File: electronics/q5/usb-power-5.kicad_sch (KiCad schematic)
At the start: 4 parts, among them U2 Li-ion charger, U3 3.20481V adjustable LDO, U7 System soft-power latch switch

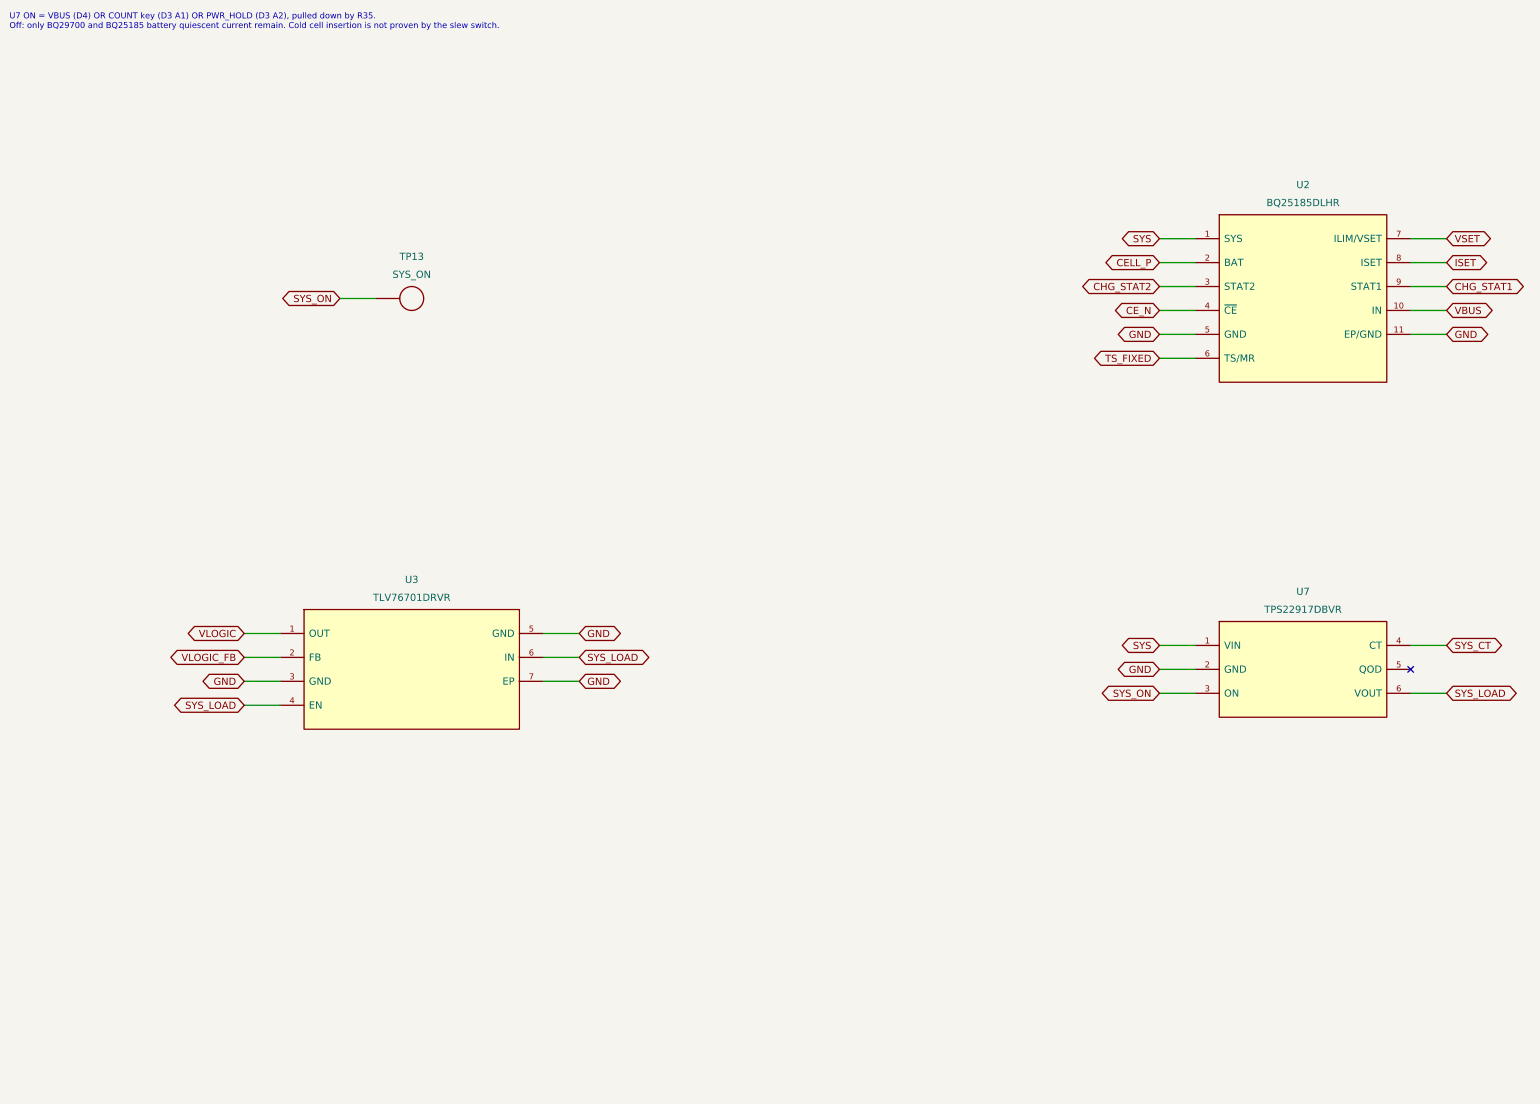
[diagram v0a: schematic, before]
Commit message: WIP: Q5 design-lock routing iteration snapshot (not verified)
Co-Authored-By: Claude Opus 5.5 <noreply@anthropic.com>
Claude-Session: https://claude.ai/code/session_01UrkzLMrBi6iLPSL5SbMCA7
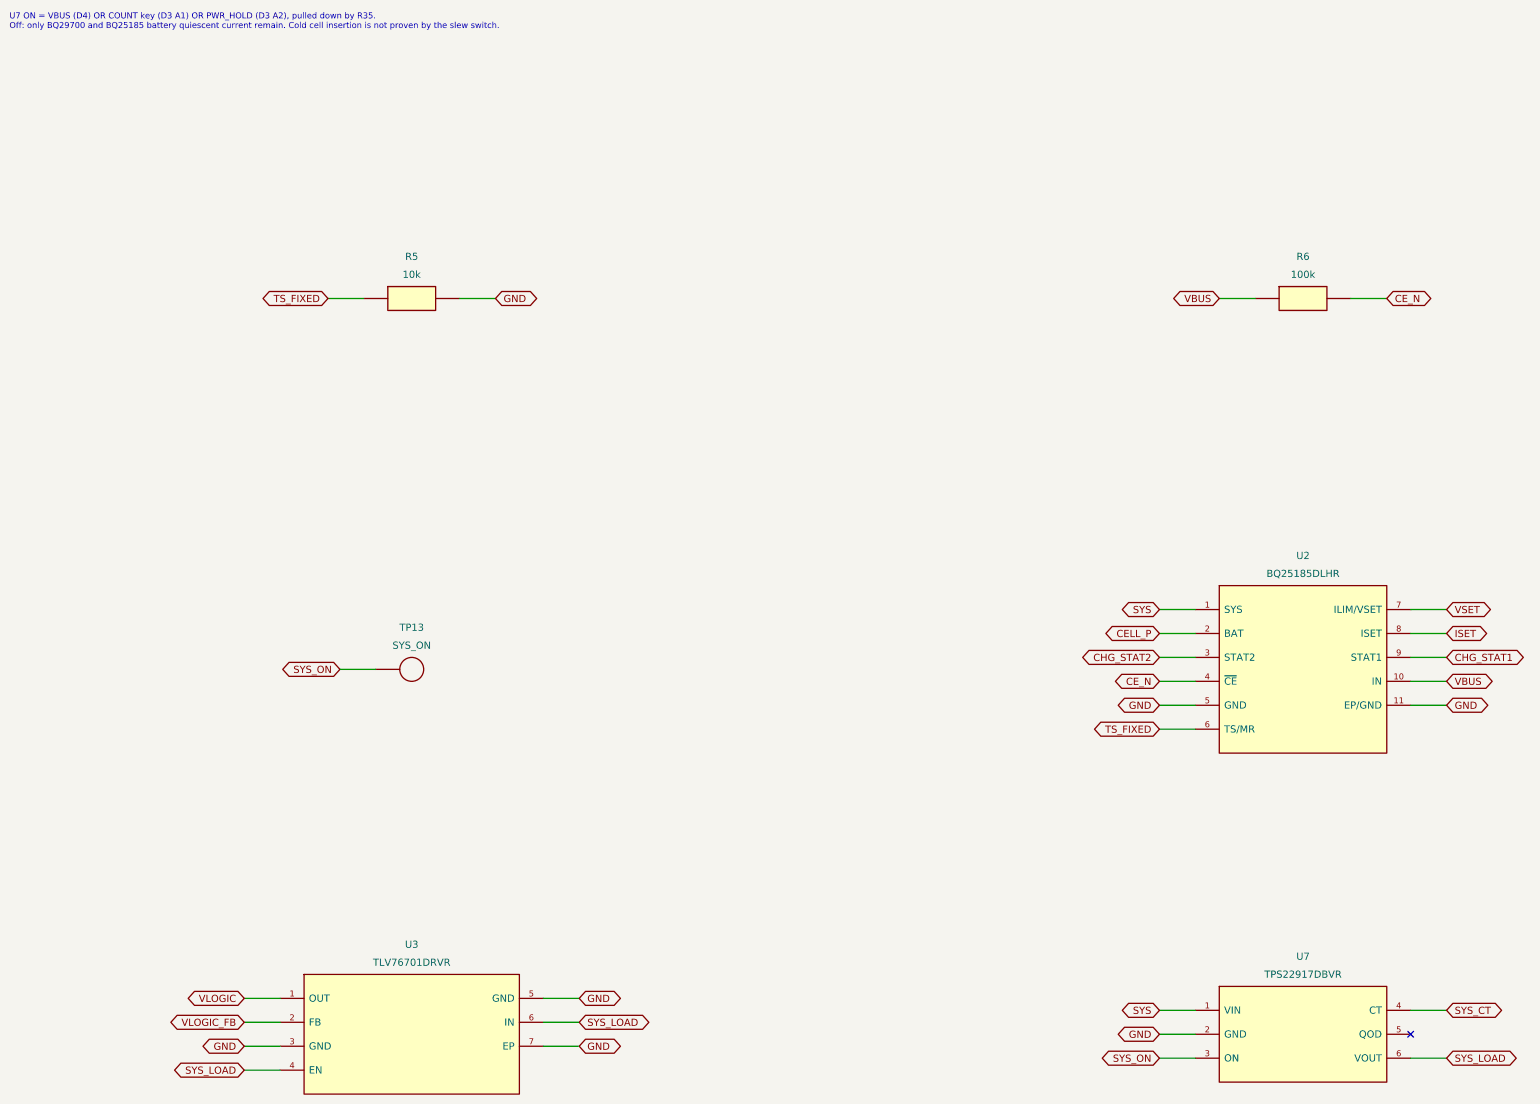
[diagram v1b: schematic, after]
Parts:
- added R5: 10k, CountFidgetQ5:Resistor_SMD_R_0603_1608Metric, symbol CountFidgetQ5:R5
- added R6: 100k, CountFidgetQ5:Resistor_SMD_R_0603_1608Metric, symbol CountFidgetQ5:R6
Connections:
- net CE_N: now also R6.2
- net GND: now also R5.2
- net TS_FIXED: now also R5.1
- net VBUS: now also R6.1
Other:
- moved on the sheet: TP13, U2, U3, U7

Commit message: Q5 design lock: JLC Basic substitutions, re-verified board, cost estimator
Co-Authored-By: Claude Opus 5.5 <noreply@anthropic.com>
Claude-Session: https://claude.ai/code/session_01UrkzLMrBi6iLPSL5SbMCA7
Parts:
- R5: MPN RC0603FR-0710KL -> 0603WAF1002T5E
- R6: MPN RC0603FR-07100KL -> 0603WAF1003T5E
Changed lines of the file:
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@@
       (in_bom yes) (on_board yes) (dnp no)
  (property "Reference" "R5" (at 105.41 73.66 0) (effects (font (size 1.524 1.524)))) (property "Value" "10k" (at 105.41 77.46999999999998 0) (effects (font (size 1.524 1.524))))
-      (property "Footprint" "CountFidgetQ5:Resistor_SMD_R_0603_1608Metric" (at 105.41 82.55 0) (effects (font (size 1.27 1.27)) (hide yes))) (property "MPN" "RC0603FR-0710KL" (at 105.41 77.46999999999998 0) (effects (font (size 1.524 1.524)) (hide yes)))
+      (property "Footprint" "CountFidgetQ5:Resistor_SMD_R_0603_1608Metric" (at 105.41 82.55 0) (effects (font (size 1.27 1.27)) (hide yes))) (property "MPN" "0603WAF1002T5E" (at 105.41 77.46999999999998 0) (effects (font (size 1.524 1.524)) (hide yes)))
       (property "Description" "1%, 0603, 0.1 W" (at 105.41 82.55 0) (effects (font (size 1.27 1.27)) (hide yes)))
       (pin "1")(pin "2")
@@
       (in_bom yes) (on_board yes) (dnp no)
  (property "Reference" "R6" (at 294.64 73.66 0) (effects (font (size 1.524 1.524)))) (property "Value" "100k" (at 294.64 77.46999999999998 0) (effects (font (size 1.524 1.524))))
-      (property "Footprint" "CountFidgetQ5:Resistor_SMD_R_0603_1608Metric" (at 294.64 82.55 0) (effects (font (size 1.27 1.27)) (hide yes))) (property "MPN" "RC0603FR-07100KL" (at 294.64 77.46999999999998 0) (effects (font (size 1.524 1.524)) (hide yes)))
+      (property "Footprint" "CountFidgetQ5:Resistor_SMD_R_0603_1608Metric" (at 294.64 82.55 0) (effects (font (size 1.27 1.27)) (hide yes))) (property "MPN" "0603WAF1003T5E" (at 294.64 77.46999999999998 0) (effects (font (size 1.524 1.524)) (hide yes)))
       (property "Description" "1%, 0603, 0.1 W" (at 294.64 82.55 0) (effects (font (size 1.27 1.27)) (hide yes)))
       (pin "1")(pin "2")
